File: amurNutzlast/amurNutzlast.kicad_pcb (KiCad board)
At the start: 4 copper layers, 125.6 x 39 mm, 97 parts, among them J1 Conn_01x06, J2 Conn_02x02_Counter_Clockwise, J4 Conn_01x08, J5 Conn_01x07, J6 USB_A, J7 Conn_01x07, J8 Conn_01x20, U1 ICE40HX1K-TQ144, U4 FT2232HL, U5 93LCxxA, U6 W25Q128JVS, U7 LD1117S33TR_SOT223, X1 SG-7050CAN, Y1 Crystal_GND24_Small

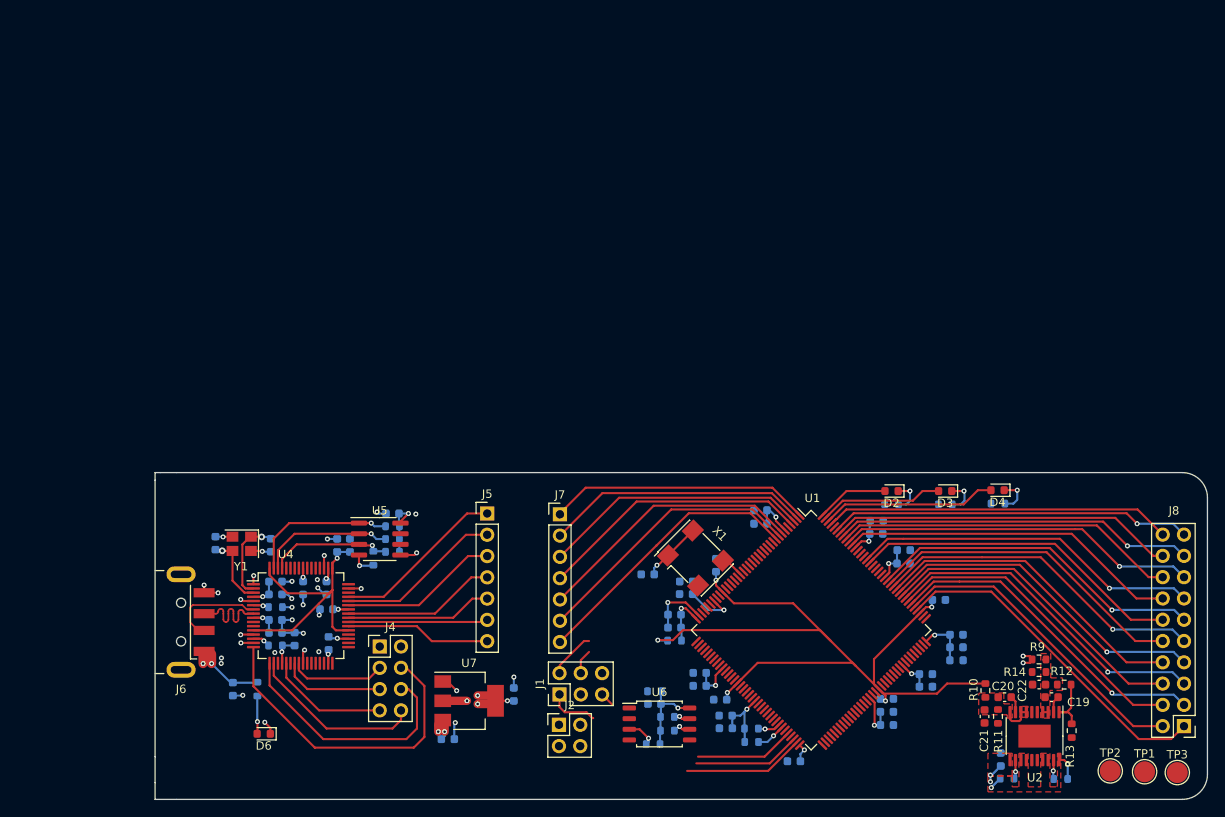
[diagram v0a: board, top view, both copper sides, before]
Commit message: finished pcb
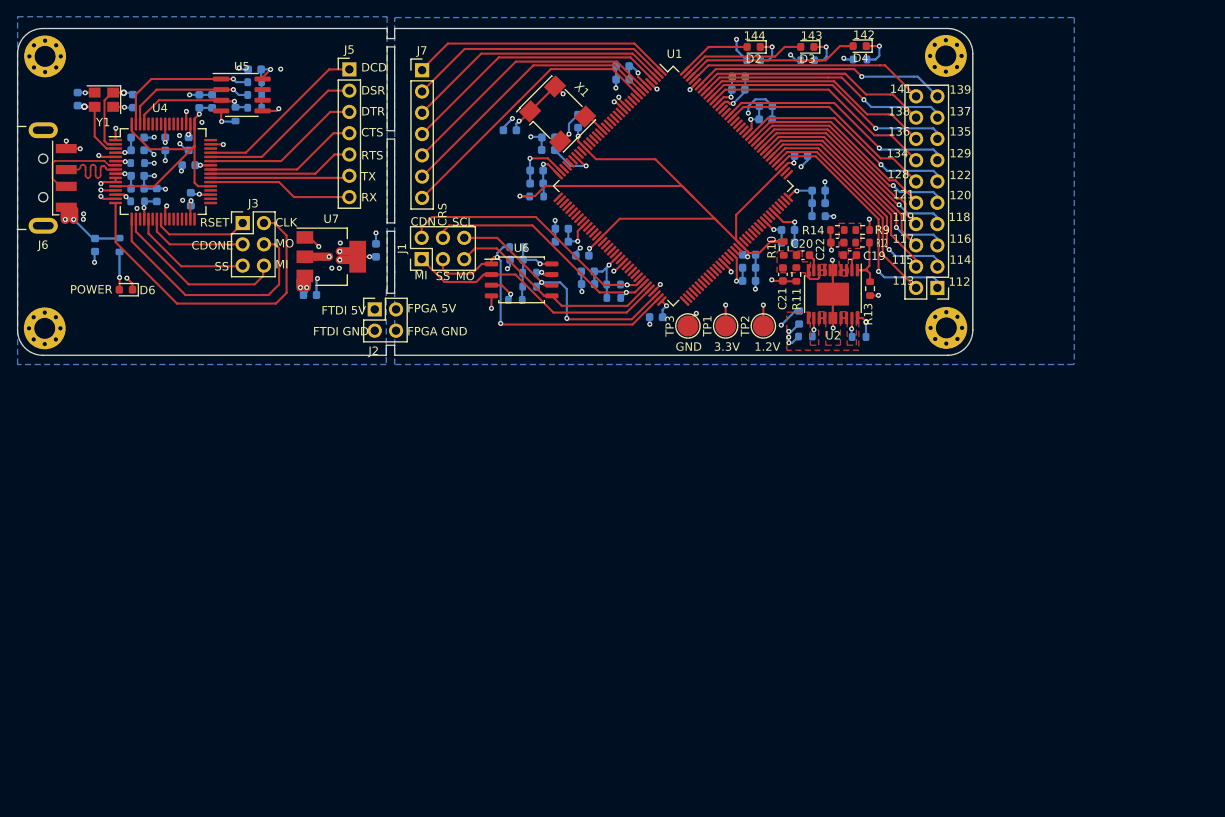
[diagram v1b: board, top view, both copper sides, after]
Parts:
- removed J4: Conn_01x08, Connector_PinHeader_2.54mm:PinHeader_2x04_P2.54mm_Vertical
- added H1: MountingHole_Pad, MountingHole:MountingHole_2.5mm_Pad_Via, F.Cu at (160.8, 33.3)
- added H2: MountingHole_Pad, MountingHole:MountingHole_2.5mm_Pad_Via, F.Cu at (53.3, 33.3)
- added H3: MountingHole_Pad, MountingHole:MountingHole_2.5mm_Pad_Via, F.Cu at (53.2, 65.8)
- added H5: MountingHole_Pad, MountingHole:MountingHole_2.5mm_Pad_Via, F.Cu at (160.8, 65.7)
- added J3: Conn_01x06, Connector_PinHeader_2.54mm:PinHeader_2x03_P2.54mm_Vertical, F.Cu at (76.9, 53.2)
- moved TP3 79.1 mm to (130.0, 65.5), turned to 90 degrees
- moved TP1 73.0 mm to (134.5, 65.5), turned to 90 degrees
- moved TP2 67.3 mm to (139.0, 65.5), turned to 90 degrees
- moved J8 60.0 mm to (159.8, 61.0)
- moved C23 58.0 mm to (143.3, 64.5)
- moved C19 58.0 mm to (149.3, 57.0)
- moved C20 58.0 mm to (143.7, 57.0)
- moved C22 58.0 mm to (147.8, 55.5)
- moved R10 58.0 mm to (141.4, 56.2)
- moved R12 58.0 mm to (150.8, 55.5)
- moved R13 58.0 mm to (151.7, 61.0)
- moved R14 58.0 mm to (147.8, 54.0)
- moved R7 58.0 mm to (150.4, 66.8)
- moved R8 58.0 mm to (144.0, 66.8)
- moved U2 58.0 mm to (147.3, 61.7)
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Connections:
- J1 pad 1: /ICE_CREST -> /MISO
- J1 pad 3: /MISO -> /SS
- J1 pad 4: /MOSI -> /ICE_CREST
- J1 pad 5: /SCL -> /MOSI
- J1 pad 6: /SS -> /SCL
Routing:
- net GND: track 0.00 -> 87.7 mm, vias 0 -> 33
- net /SS: track 14.5 -> 39.7 mm, vias 0 -> 2
- net /ICE_CDONE: track 8.38 -> 32.4 mm
- net /MOSI: track 2.94 -> 26.2 mm
- net /ICE_CREST: track 9.60 -> 29.8 mm
- net /MISO: track 11.9 -> 31.8 mm
- net /SCL: track 16.8 -> 32.3 mm, vias 1 -> 2
- net /fpga/PIO10: track 38.4 -> 24.5 mm
- net /fpga/PIO11: track 40.5 -> 26.9 mm
- net /fpga/PIO9: track 40.2 -> 26.8 mm
- net /fpga/PIO7: track 40.1 -> 26.7 mm
- net /fpga/PIO12: track 39.6 -> 26.2 mm
- net /fpga/PIO8: track 38.2 -> 24.9 mm
- net /fpga/PIO13: track 41.8 -> 28.8 mm
- net /fpga/PIO6: track 38.0 -> 25.3 mm
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- added copper zone on B.Cu, net GND
- added copper zone on In1.Cu, net GND
- added copper zone on B.Cu, net GND1
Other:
- board size 125.6 x 39 mm -> 114 x 39 mm
- board text added: "1.2V"
- board text added: "112"
- board text added: "113"
- board text added: "114"
- board text added: "115"
- board text added: "116"
- board text added: "117"
- board text added: "118"
- board text added: "119"
- board text added: "120"
- board text added: "121"
- board text added: "122"
- board text added: "128"
- board text added: "129"
- board text added: "134"
- board text added: "135"
- board text added: "136"
- board text added: "137"
- board text added: "138"
- board text added: "139"
- board text added: "141"
- board text added: "142"
- board text added: "143"
- board text added: "144"
- board text added: "3.3V"
- board text added: "CDN"
- board text added: "CDONE"
- board text added: "CLK"
- board text added: "CRS"
- board text added: "CTS"
- board text added: "DCD"
- board text added: "DSR"
- board text added: "DTR"
- board text added: "FPGA 5V"
- board text added: "FPGA GND"
- board text added: "FTDI 5V"
- board text added: "FTDI GND"
- board text added: "GND"
- board text added: "MI"
- board text added: "MO"
- board text added: "POWER"
- board text added: "RSET"
- board text added: "RTS"
- board text added: "RX"
- board text added: "SCL"
- board text added: "SS"
- board text added: "TX"
